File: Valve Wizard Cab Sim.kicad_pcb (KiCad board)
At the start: 2 copper layers, 73 x 74 mm, 48 parts, among them J1 IN, J2 FS_5, J3 Power, J4 Battery, J5 FS4, J6 GND, J7 OUT_S, Q1 BC337, Q2 BC327, Q3 BS170, U1 TL072

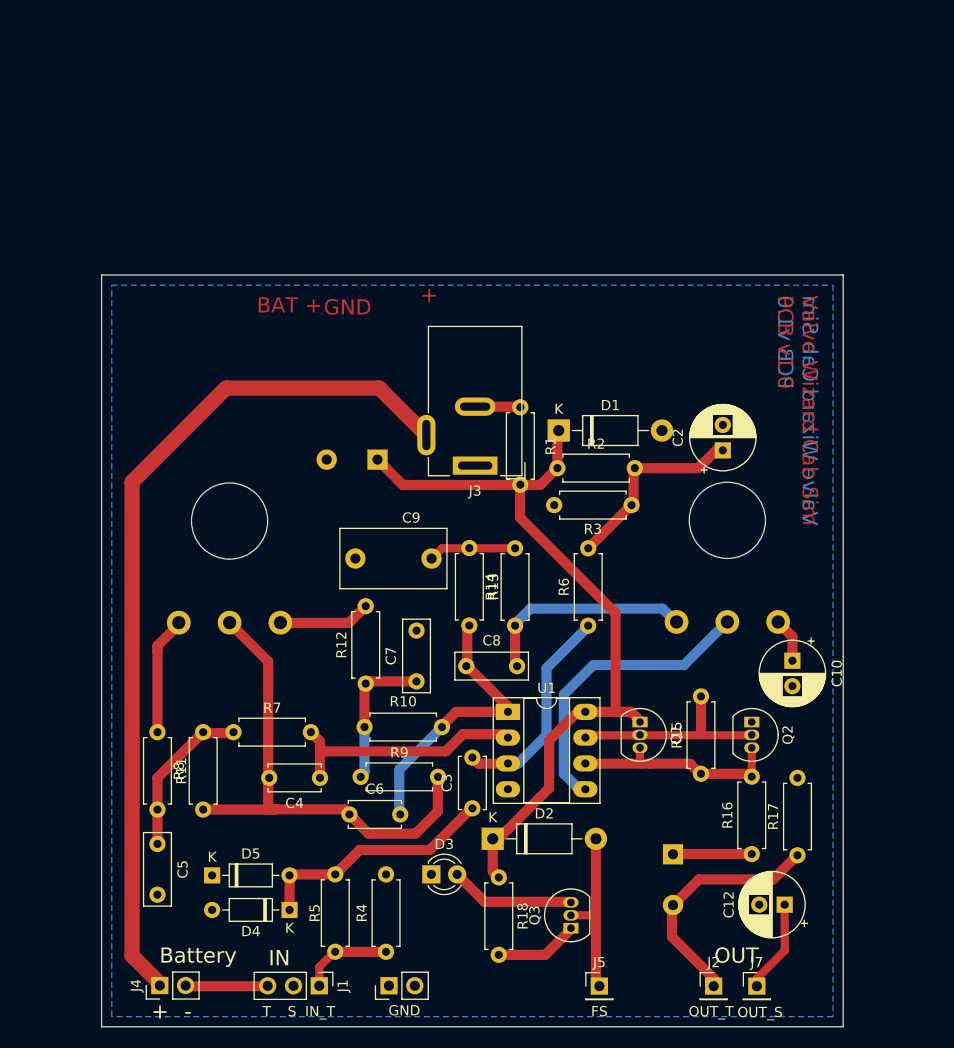
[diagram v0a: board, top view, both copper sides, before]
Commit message: new
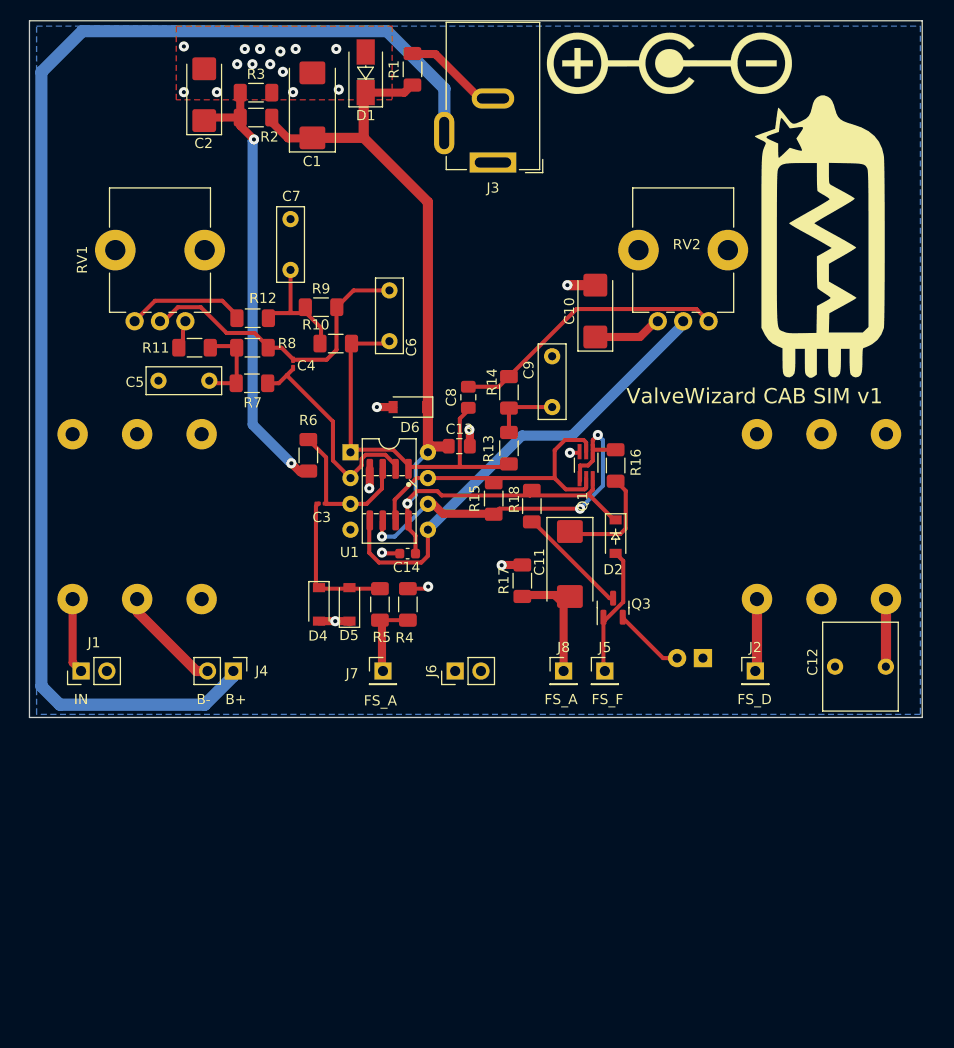
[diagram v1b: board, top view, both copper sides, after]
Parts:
- removed Q2: BC327, Package_TO_SOT_THT:TO-92_Inline
- added C13: 100n, Capacitor_SMD:C_0805_2012Metric_Pad1.18x1.45mm_HandSolder, F.Cu at (74.2, 73.8)
- added C14: 100n, Capacitor_SMD:C_0603_1608Metric, F.Cu at (69.1, 84.4)
- added D6: BZT52Bxx, Diode_SMD:D_SOD-123, F.Cu at (69.3, 70.0)
- added J10: IN, Connector_Audio:Jack_6.35mm_Neutrik_NMJ6HCD2_Horizontal, B.Cu at (36.1, 88.9)
- added J11: IN, Connector_Audio:Jack_6.35mm_Neutrik_NMJ6HCD2_Horizontal, B.Cu at (103.5, 88.9)
- added J8: FS_E, Connector_PinHeader_2.54mm:PinHeader_1x01_P2.54mm_Vertical, F.Cu at (84.5, 96.0)
- added REF**: ValveWizard, MyLibraries:ValveWizard, F.Cu at (110.0, 53.3)
- added REF**: Polarity_Center_Negative_6mm_SilkScreen, Symbol:Polarity_Center_Negative_6mm_SilkScreen, F.Cu at (94.9, 36.2)
- added REF**: ValveWizard, MyLibraries:ValveWizard, B.Cu at (109.8, 53.4)
- C1, C11: footprint Capacitor_THT:CP_Radial_D10.0mm_P5.00mm -> Capacitor_Tantalum_SMD:CP_EIA-7343-43_Kemet-X_Pad2.25x2.55mm_HandSolder; moved to F.Cu
- C10, C2: footprint Capacitor_THT:CP_Radial_D6.3mm_P2.50mm -> Capacitor_Tantalum_SMD:CP_EIA-6032-28_Kemet-C_Pad2.25x2.35mm_HandSolder
- C12: footprint Capacitor_THT:CP_Radial_D6.3mm_P2.50mm -> Capacitor_THT:C_Rect_L7.2mm_W8.5mm_P5.00mm_FKP2_FKP2_MKS2_MKP2
- C3, C4: footprint Capacitor_THT:C_Disc_D5.0mm_W2.5mm_P5.00mm -> Capacitor_SMD:C_0201_0603Metric_Pad0.64x0.40mm_HandSolder
- C5, C7: footprint Capacitor_THT:C_Disc_D7.0mm_W2.5mm_P5.00mm -> Capacitor_THT:C_Rect_L7.2mm_W2.5mm_P5.00mm_FKS2_FKP2_MKS2_MKP2
- C6: footprint Capacitor_THT:C_Disc_D5.0mm_W2.5mm_P5.00mm -> Capacitor_THT:C_Rect_L7.2mm_W2.5mm_P5.00mm_FKS2_FKP2_MKS2_MKP2
- C8: footprint Capacitor_THT:C_Disc_D7.0mm_W2.5mm_P5.00mm -> Capacitor_SMD:C_0805_2012Metric_Pad1.18x1.45mm_HandSolder
- C9: footprint Capacitor_THT:C_Rect_L10.3mm_W5.7mm_P7.50mm_MKS4 -> Capacitor_THT:C_Rect_L7.2mm_W2.5mm_P5.00mm_FKS2_FKP2_MKS2_MKP2
- D1: footprint Diode_THT:D_DO-41_SOD81_P10.16mm_Horizontal -> Diode_SMD:D_SMA
- D2: value 1n4001 -> 1n4148; footprint Diode_THT:D_DO-41_SOD81_P10.16mm_Horizontal -> Diode_SMD:D_SOD-123
- D3: moved to B.Cu
- D4, D5: footprint Diode_THT:D_DO-35_SOD27_P7.62mm_Horizontal -> Diode_SMD:D_SOD-123
- J1: footprint Connector_PinHeader_2.54mm:PinHeader_1x03_P2.54mm_Vertical -> Connector_PinHeader_2.54mm:PinHeader_1x02_P2.54mm_Vertical
- J2: value FS_5 -> FS
- J3: footprint Connector_BarrelJack:BarrelJack_Wuerth_6941xx301002 -> Connector_BarrelJack:BarrelJack_GCT_DCJ200-10-A_Horizontal
- J5: value FS4 -> FS_F
- J7: value OUT_S -> FS
- Q1: value BC337 -> MMDT3946; footprint Package_TO_SOT_THT:TO-92_Inline -> Package_TO_SOT_SMD:SOT-363_SC-70-6_Handsoldering
- Q3: value BS170 -> MMBF170; footprint Package_TO_SOT_THT:TO-92_Inline -> Package_TO_SOT_SMD:SOT-23
- R1, R10, R12, R13, R15, R16, R2, R3, R4, R5, R6, R9: footprint Resistor_THT:R_Axial_DIN0207_L6.3mm_D2.5mm_P7.62mm_Horizontal -> Resistor_SMD:R_1206_3216Metric_Pad1.30x1.75mm_HandSolder
- R11: value 1k -> 1K; footprint Resistor_THT:R_Axial_DIN0207_L6.3mm_D2.5mm_P7.62mm_Horizontal -> Resistor_SMD:R_1206_3216Metric_Pad1.30x1.75mm_HandSolder
- R14: value 33k -> 33K; footprint Resistor_THT:R_Axial_DIN0207_L6.3mm_D2.5mm_P7.62mm_Horizontal -> Resistor_SMD:R_1206_3216Metric_Pad1.30x1.75mm_HandSolder
- R17, R7: value 10k -> 10K; footprint Resistor_THT:R_Axial_DIN0207_L6.3mm_D2.5mm_P7.62mm_Horizontal -> Resistor_SMD:R_1206_3216Metric_Pad1.30x1.75mm_HandSolder
- R18: value 4k7 -> 4K7; footprint Resistor_THT:R_Axial_DIN0207_L6.3mm_D2.5mm_P7.62mm_Horizontal -> Resistor_SMD:R_1206_3216Metric_Pad1.30x1.75mm_HandSolder
- R8: value 22k -> 22K; footprint Resistor_THT:R_Axial_DIN0207_L6.3mm_D2.5mm_P7.62mm_Horizontal -> Resistor_SMD:R_1206_3216Metric_Pad1.30x1.75mm_HandSolder
- RV1: value CAB 100K -> 100KB; footprint Potentiometer_THT:Potentiometer_Piher_T-16L_Single_Vertical_Hole -> Potentiometer_THT:Potentiometer_Bourns_PTV09A-1_Single_Vertical; moved to F.Cu
- RV2: footprint Potentiometer_THT:Potentiometer_Piher_T-16L_Single_Vertical_Hole -> Potentiometer_THT:Potentiometer_Bourns_PTV09A-1_Single_Vertical; moved to F.Cu
- U1: footprint Package_DIP:DIP-8_W7.62mm_Socket_LongPads -> MyLibraries:SOIC_DIP-8
- moved C2 61.9 mm to (49.1, 39.2)
- moved R3 54.9 mm to (54.2, 39.0), turned to 0 degrees
- moved C6 51.7 mm to (67.3, 58.5), turned to -90 degrees
- moved J7 48.1 mm to (66.7, 96.0)
- moved R9 46.4 mm to (60.6, 60.2)
- moved C5 45.9 mm to (49.6, 67.4), turned to 180 degrees
- moved R8 45.7 mm to (53.9, 64.2), turned to 180 degrees
- moved R2 45.5 mm to (54.2, 41.5), turned to 180 degrees
- moved C7 42.4 mm to (57.6, 56.5)
- moved R1 42.2 mm to (69.6, 36.8)
- moved C4 40.8 mm to (57.9, 65.8), turned to 90 degrees
- moved R16 40.5 mm to (89.6, 75.8)
- moved D1 40.1 mm to (65.0, 37.0), turned to 90 degrees
- moved C10 39.5 mm to (87.6, 60.5), turned to 90 degrees
- moved R10 39.2 mm to (62.0, 63.8)
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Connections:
- net Net-(J3-Pad2) renamed VIN
- net Net-(J3-Pad3) renamed BAT+
- C1 pad 2: IN_S -> GND
- C10 pad 2: IN_S -> GND
- C11 pad 2: FS_IN2 -> FS_E
- C12 pad 2: IN_S -> GND
- C2 pad 2: IN_S -> GND
- C5 pad 2: IN_S -> GND
- C7 pad 2: IN_S -> GND
- C9 pad 2: IN_S -> GND
- D1 pad 2: IN_S -> GND
- D2 pad 2: FS_NC2 -> FS_F
- D3 pad 1: IN_S -> GND
- D4 pad 2: IN_S -> GND
- D5 pad 1: IN_S -> GND
- J1 pad 1: FS_IN -> IN_T
- J1 pad 2: IN_S -> GND
- J2 pad 1: FS_IN2 -> FS_CD
- J3 pad 1: IN_S -> GND
- J4 pad 2: IN_R -> BAT-
- J5 pad 1: FS_NC2 -> FS_F
- J6 pad 1: IN_S -> GND
- J6 pad 2: IN_S -> GND
- J7 pad 1: Net-(C12-Pad1) -> FS_A
- Q1 pad 1: 9V -> Net-(Q1-Pad1)
- Q1 pad 3: Net-(Q1-Pad3) -> GND
- Q3 pad 1: Net-(Q3-Pad1) -> FS_F
- Q3 pad 2: FS_NC2 -> Net-(D3-Pad2)
- Q3 pad 3: Net-(D3-Pad2) -> Net-(Q3-Pad3)
- R15 pad 1: Net-(Q1-Pad3) -> Net-(Q1-Pad1)
- R16 pad 2: Net-(Q1-Pad3) -> Net-(Q1-Pad1)
- R17 pad 1: FS_IN2 -> FS_E
- R17 pad 2: IN_S -> GND
- R18 pad 2: Net-(Q3-Pad1) -> Net-(Q3-Pad3)
- R3 pad 2: IN_S -> GND
- R4 pad 1: FS_IN -> FS_A
- R4 pad 2: IN_S -> GND
- R5 pad 2: FS_IN -> FS_A
- U1 pad 4: IN_S -> GND
- U1 pad 6: Net-(Q1-Pad3) -> Net-(Q1-Pad1)
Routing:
- net BAT+: track 84.8 -> 130.0 mm
- net Net-(Q1-Pad1): track 0.00 -> 39.2 mm, vias 0 -> 3
- net 4.5V: track 19.3 -> 44.6 mm, vias 0 -> 2
- net FS_IN2: track 24.0 -> 0.00 mm
- net Net-(Q1-Pad3): track 21.2 -> 0.00 mm
- net Net-(C4-Pad2): track 49.4 -> 31.0 mm
- net GND: track 0.00 -> 17.6 mm, vias 0 -> 23
- net FS_NC2: track 17.3 -> 0.00 mm
- net Net-(RV2-Pad2): track 29.4 -> 46.1 mm
- net 9V: track 76.2 -> 91.5 mm, vias 0 -> 1
- net FS_F: track 0.00 -> 13.2 mm
- net FS_E: track 0.00 -> 12.6 mm
- net Net-(Q3-Pad3): track 0.00 -> 11.1 mm
- net BAT-: track 0.00 -> 10.7 mm
- net Net-(C6-Pad2): track 27.4 -> 37.9 mm
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- added copper zone on B.Cu, net GND
- added copper zone on F.Cu, net GND
- removed copper zone on B.Cu, net IN_S
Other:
- board size 73 x 74 mm -> 87.9 x 68.6 mm
- net class Default removed
- board text added: "B+"
- board text added: "B-"
- board text added: "FS_A"
- board text added: "FS_D"
- board text added: "FS_F"
- board text added: "IN"
- board text added: "ValveWizard CAB SIM v1"
- board text removed: "+"
- board text removed: "-"
- board text removed: "BAT +"
- board text removed: "FS"
- board text removed: "GND"
- board text removed: "IN_T"
- board text removed: "OUT"
- board text removed: "OUT_T"
- board text removed: "S"
- board text removed: "T"
- board text removed: "Valve Wizard Cab Sim PCB v1.0"

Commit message: latest
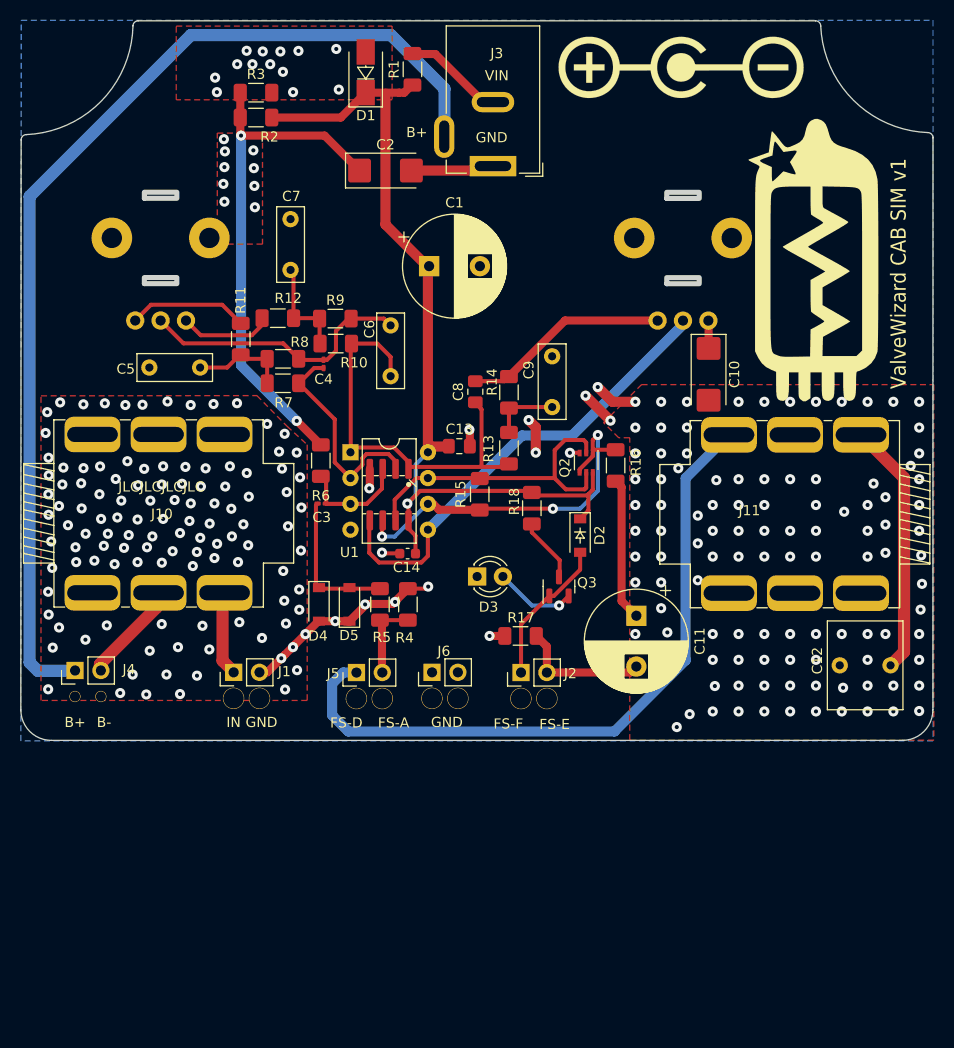
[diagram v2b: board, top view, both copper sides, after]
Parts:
- removed D6: BZT52Bxx, Diode_SMD:D_SOD-123
- removed J7: FS, Connector_PinHeader_2.54mm:PinHeader_1x01_P2.54mm_Vertical
- removed J8: FS_E, Connector_PinHeader_2.54mm:PinHeader_1x01_P2.54mm_Vertical
- removed Q1: MMDT3946, Package_TO_SOT_SMD:SOT-363_SC-70-6_Handsoldering
- added Q2: BC846BPN, Package_TO_SOT_SMD:SOT-363_SC-70-6, F.Cu at (86.7, 75.5)
- C1, C11: footprint Capacitor_Tantalum_SMD:CP_EIA-7343-43_Kemet-X_Pad2.25x2.55mm_HandSolder -> Capacitor_THT:CP_Radial_D10.0mm_P5.00mm
- J1, J4, J6: footprint Connector_PinHeader_2.54mm:PinHeader_1x02_P2.54mm_Vertical -> Wire_Connector_Supported:PinHeader_1x02_P2.54mm_Vertical
- J10: footprint Connector_Audio:Jack_6.35mm_Neutrik_NMJ6HCD2_Horizontal -> MyLibraries:Jack_6.35mm_Neutrik_NMJ6HC-S_SOLDER_LUG; moved to F.Cu
- J11: value IN -> OUT; footprint Connector_Audio:Jack_6.35mm_Neutrik_NMJ6HCD2_Horizontal -> MyLibraries:Jack_6.35mm_Neutrik_NMJ6HC-S_SOLDER_LUG; moved to F.Cu
- J2: value FS -> FS_EF; footprint Connector_PinHeader_2.54mm:PinHeader_1x01_P2.54mm_Vertical -> Wire_Connector_Supported:PinHeader_1x02_P2.54mm_Vertical
- J5: value FS_F -> FS; footprint Connector_PinHeader_2.54mm:PinHeader_1x01_P2.54mm_Vertical -> Wire_Connector_Supported:PinHeader_1x02_P2.54mm_Vertical
- RV1, RV2: moved to B.Cu
- moved D3 23.6 mm to (76.0, 86.7), turned to 0 degrees
- moved J5 23.3 mm to (65.3, 97.6), turned to 90 degrees
- moved J2 21.9 mm to (81.5, 97.6), turned to 90 degrees
- moved C1 19.6 mm to (71.2, 56.1), turned to 0 degrees
- moved C2 19.3 mm to (66.9, 46.7), turned to 0 degrees
- moved J1 16.4 mm to (53.2, 97.6)
- moved J4 14.4 mm to (37.6, 97.4), turned to 90 degrees
- moved C10 12.8 mm to (98.8, 66.8), turned to -90 degrees
- moved J10 11.9 mm to (44.6, 80.5)
- moved J11 9.19 mm to (107.3, 80.5), turned to 180 degrees
- moved C11 8.29 mm to (91.6, 90.5)
- moved Q3 5.72 mm to (84.0, 87.7)
- moved R17 5.44 mm to (80.2, 92.5), turned to 180 degrees
- moved RV2 5.01 mm to (93.7, 61.5)
- moved RV1 4.94 mm to (42.3, 61.5)
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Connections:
- net Net-(C12-Pad1) renamed /Sleeve
- J10 pad RN: unconnected-(J10-PadRN) -> GND
- J10 pad SN: unconnected-(J10-PadSN) -> GND
- J11 pad RN: unconnected-(J11-PadRN) -> GND
- J11 pad SN: unconnected-(J11-PadSN) -> GND
- J11 pad TN: unconnected-(J11-PadTN) -> GND
- J2 pad 1: FS_CD -> FS_F
- J5 pad 1: FS_F -> FS_CD
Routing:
- net FS_CD: track 7.18 -> 68.3 mm
- net GND: track 17.6 -> 50.4 mm, vias 23 -> 259
- net BAT+: track 130.0 -> 104.8 mm
- net /Sleeve: track 6.66 -> 25.0 mm
- net Net-(R11-Pad1): track 2.72 -> 11.8 mm
- net Net-(C8-Pad2): track 27.3 -> 20.4 mm
- net 4.5V: track 44.6 -> 51.1 mm
- net Net-(Q3-Pad3): track 11.1 -> 6.37 mm
- net Net-(C3-Pad2): track 15.2 -> 11.1 mm
- net Net-(C10-Pad1): track 6.66 -> 2.75 mm
- net Net-(C4-Pad2): track 31.0 -> 27.4 mm
- net Net-(C6-Pad2): track 37.9 -> 41.0 mm
- net Net-(C11-Pad1): track 11.1 -> 14.1 mm
- net Net-(C7-Pad1): track 12.8 -> 10.1 mm
- net Net-(R12-Pad2): track 11.9 -> 9.18 mm
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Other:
- board size 87.9 x 68.6 mm -> 89.8 x 70.8 mm
- board text added: "D3"
- board text added: "FS-A"
- board text added: "FS-D"
- board text added: "FS-E"
- board text added: "FS-F"
- board text added: "GND"
- board text added: "JLCJLCJLCJLC"
- board text added: "VIN"
- board text removed: "FS_A"
- board text removed: "FS_D"
- board text removed: "FS_F"
